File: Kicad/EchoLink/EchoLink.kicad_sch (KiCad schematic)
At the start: 37 parts, among them U1 STM32L433CCT6

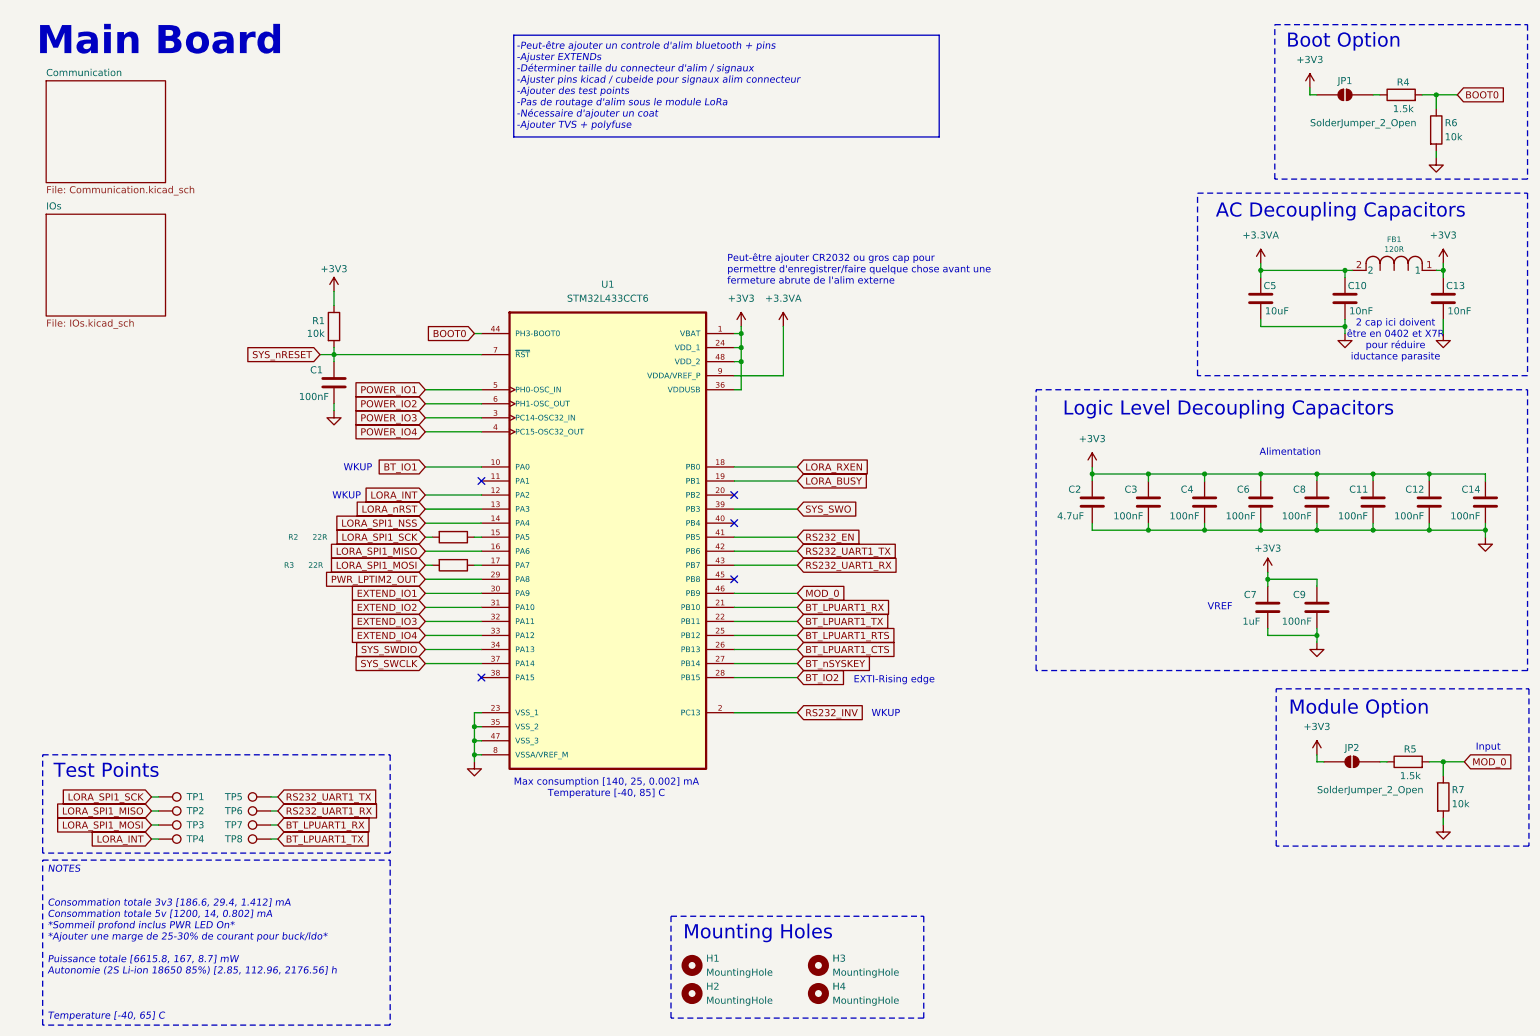
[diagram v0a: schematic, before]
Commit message: wip: connector and bms IOs
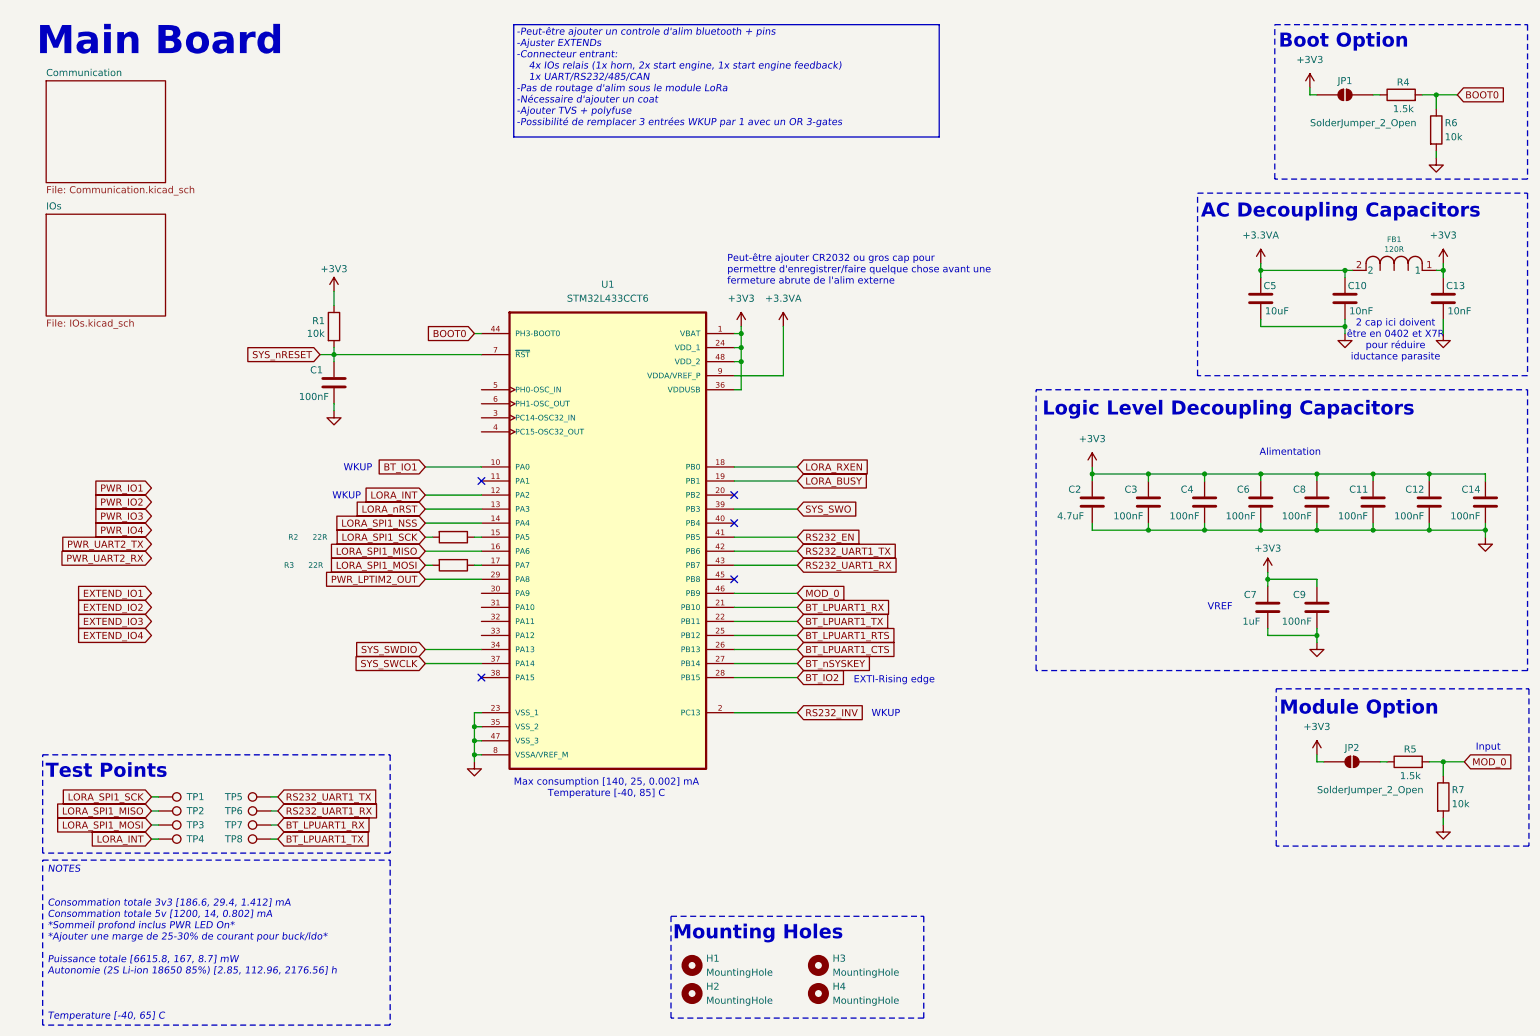
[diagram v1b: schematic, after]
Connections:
- net EXTEND_IO1: no longer U1.30 (PA9)
- net EXTEND_IO2: no longer U1.31 (PA10)
- net EXTEND_IO3: no longer U1.32 (PA11)
- net EXTEND_IO4: no longer U1.33 (PA12)
- net POWER_IO1: no longer names the net of U1.5 (PH0-OSC_IN)
- net POWER_IO2: no longer names the net of U1.6 (PH1-OSC_OUT)
- net POWER_IO3: no longer names the net of U1.3 (PC14-OSC32_IN)
- net POWER_IO4: no longer names the net of U1.4 (PC15-OSC32_OUT)
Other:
- note added: "-Peut-être ajouter un controle d'alim bluetooth + pins -Ajuster EXTENDs -Connecteur entrant: 4x IOs relais (1x horn, 2x start engine, 1x start engine feedback) 1x UART/RS232/485/CAN -Pas de routage d'alim sous le module LoRa -Nécessaire d'ajouter un coat -Ajouter TVS + polyfuse -Possibilité de remplacer 3 entrées WKUP par 1 avec un OR 3-gates"
- note removed: "-Peut-être ajouter un controle d'alim bluetooth + pins -Ajuster EXTENDs -Déterminer taille du connecteur d'alim / signaux -Ajuster pins kicad / cubeide pour signaux alim connecteur -Ajouter des test points -Pas de routage d'alim sous le module LoRa -Nécessaire d'ajouter un coat -Ajouter TVS + polyfuse"
